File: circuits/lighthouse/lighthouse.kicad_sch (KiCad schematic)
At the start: 16 parts, among them Q1 S9013, U1 DCDC_StepUp_SX1308, U2 ESP32 CP2102

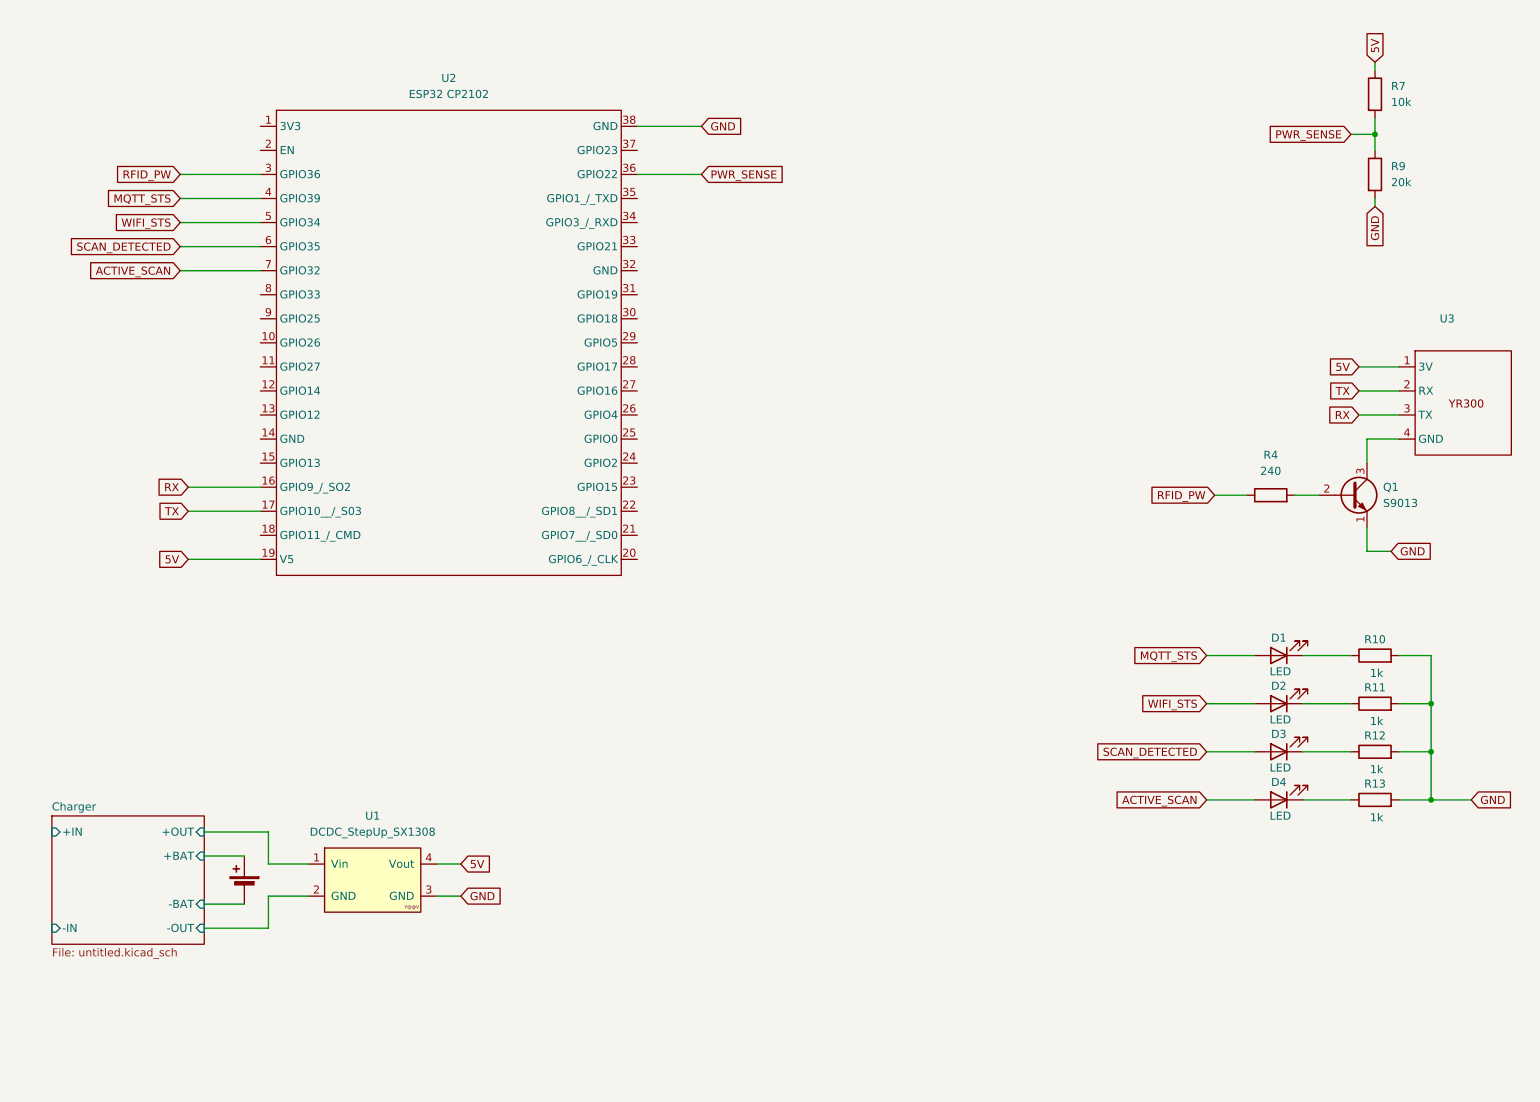
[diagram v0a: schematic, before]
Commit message: More circuits
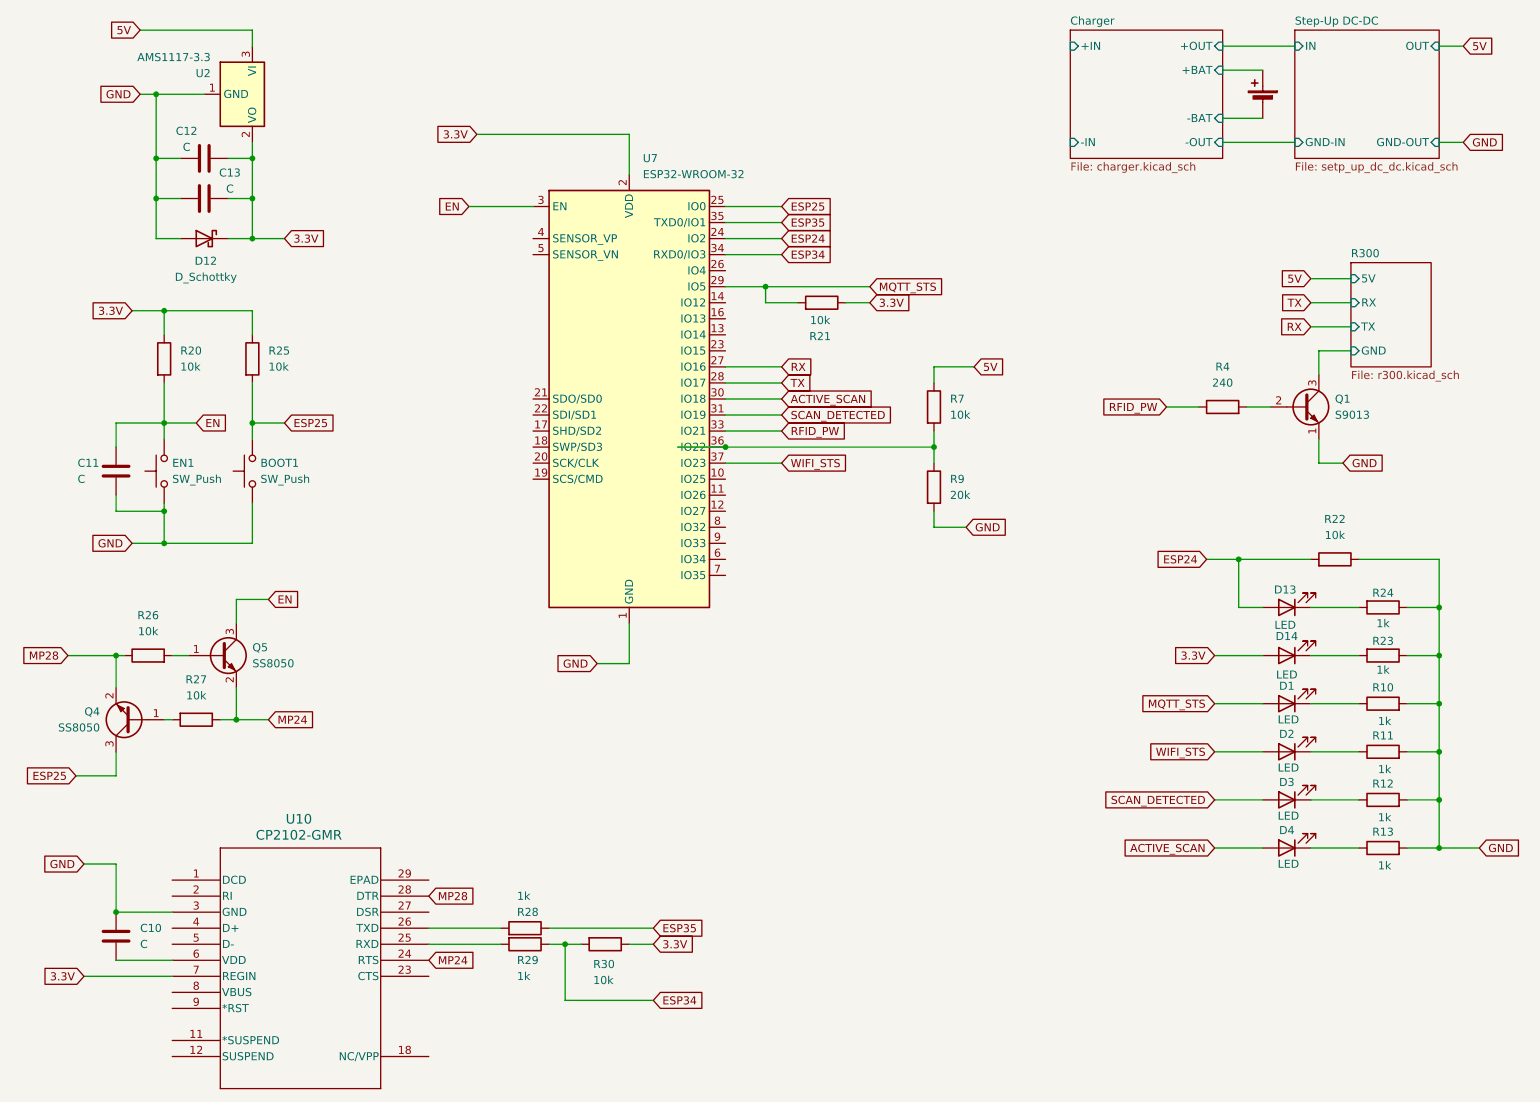
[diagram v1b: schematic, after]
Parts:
- removed U1: DCDC_StepUp_SX1308, SX1308_DCDC_boost:DCDC_StepUp_SX1308, symbol DCDC_StepUp_SX1308:DCDC_StepUp_SX1308
- removed U2: ESP32 CP2102, ESP32:ESP32_38Pin, symbol ESP32:ESP32_38Pin_Symbol
- removed U3: ~, YR300:YR300, symbol YR300:YR300
- added BOOT1, EN1: SW_Push, Button_Switch_SMD:SW_Push_SPST_NO_Alps_SKRK, symbol Switch:SW_Push
- added C10, C11, C12, C13: C, Capacitor_SMD:C_1206_3216Metric_Pad1.33x1.80mm_HandSolder, symbol Device:C
- added D12: D_Schottky, Diode_SMD:D_2114_3652Metric_Pad1.85x3.75mm_HandSolder, symbol Device:D_Schottky
- added D13, D14: LED, LED_SMD:LED_1206_3216Metric_Pad1.42x1.75mm_HandSolder, symbol Device:LED
- added Q4, Q5: SS8050, Package_TO_SOT_SMD:SOT-23, symbol Transistor_BJT:SS8050
- added R20, R21, R22, R25, R26, R27, R30: 10k, Resistor_SMD:R_1206_3216Metric_Pad1.30x1.75mm_HandSolder, symbol Device:R
- added R23, R24, R28, R29: 1k, Resistor_SMD:R_1206_3216Metric_Pad1.30x1.75mm_HandSolder, symbol Device:R
- added U10: CP2102-GMR, CP2102-GMR:QFN28_5X5_SIL, symbol CP2102-GMR:CP2102-GMR
- added U2: AMS1117-3.3, Package_TO_SOT_SMD:SOT-223-3_TabPin2, symbol Regulator_Linear:AMS1117-3.3
- added U7: ESP32-WROOM-32, RF_Module:ESP32-WROOM-32, symbol RF_Module:ESP32-WROOM-32
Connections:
- net 5V: now also U2.3 (VI)
- net ACTIVE_SCAN: now also U7.30 (IO18)
- net GND: now also BOOT1.1, C10.1, C11.2, C12.2, C13.2, D12.2 (A), EN1.1, R22.1, R23.1, R24.1, U10.3 (GND), U2.1 (GND), U7.1 (GND), U7.15 (GND), U7.38 (GND), U7.39 (GND)
- net MQTT_STS: now also R21.2, U7.29 (IO5)
- net RFID_PW: now also U7.33 (IO21)
- net RX: now also U7.27 (IO16)
- net SCAN_DETECTED: now also U7.31 (IO19)
- net TX: now also U7.28 (IO17)
- net WIFI_STS: now also U7.37 (IO23)
- net R300/GND: now reaches Q1.3 (C)
- net PWR_SENSE: no longer names the net of R7.2, R9.1
- net PWR_SENSE: now also U7.36 (IO22)
- new net: R29.2, U10.25 (RXD)
- new net: Q5.1 (B), R26.2
- new net: D13.1 (K), R24.2
- new net: C10.2, U10.6 (VDD)
- new net: R28.2, U10.26 (TXD)
- new net: D14.1 (K), R23.2
- new net: Q4.1 (B), R27.2
- new net 3.3V: C12.1, C13.1, D12.1 (K), D14.2 (A), R20.1, R21.1, R25.1, R30.1, U10.7 (REGIN), U2.2 (VO), U7.2 (VDD)
- new net EN: C11.1, EN1.2, Q5.3 (C), R20.2, U7.3 (EN)
- new net ESP24: D13.2 (A), R22.2, U7.24 (IO2)
- new net ESP25: BOOT1.2, Q4.3 (C), R25.2, U7.25 (IO0)
- new net ESP34: R29.1, R30.2, U7.34 (RXD0/IO3)
- new net ESP35: R28.1, U7.35 (TXD0/IO1)
- new net MP24: Q5.2 (E), R27.1, U10.24 (RTS)
- new net MP28: Q4.2 (E), R26.1, U10.28 (DTR)
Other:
- added sheet R300 (r300.kicad_sch)
- added sheet Step-Up DC-DC (setp_up_dc_dc.kicad_sch)
- sheet Charger: file untitled.kicad_sch -> charger.kicad_sch
- moved on the sheet: D1, D2, D3, D4, Q1, R10, R11, R12, R13, R4, R7, R9
